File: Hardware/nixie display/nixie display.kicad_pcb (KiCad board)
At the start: 2 copper layers, 99.8 x 49.6 mm, 37 parts, among them J1 Conn_01x05_Male, J2 Conn_01x03_Male, J3 Conn_01x02_Male, J4 Conn_01x02_Male, J5 Conn_01x05_Male, J6 Conn_01x02_Male, Q1 MJE13003, Q2 Q_NMOS_GSD, U1 K155ID1, U10 TLP627, U7 TLP627, U8 TLP627, U9 TLP627

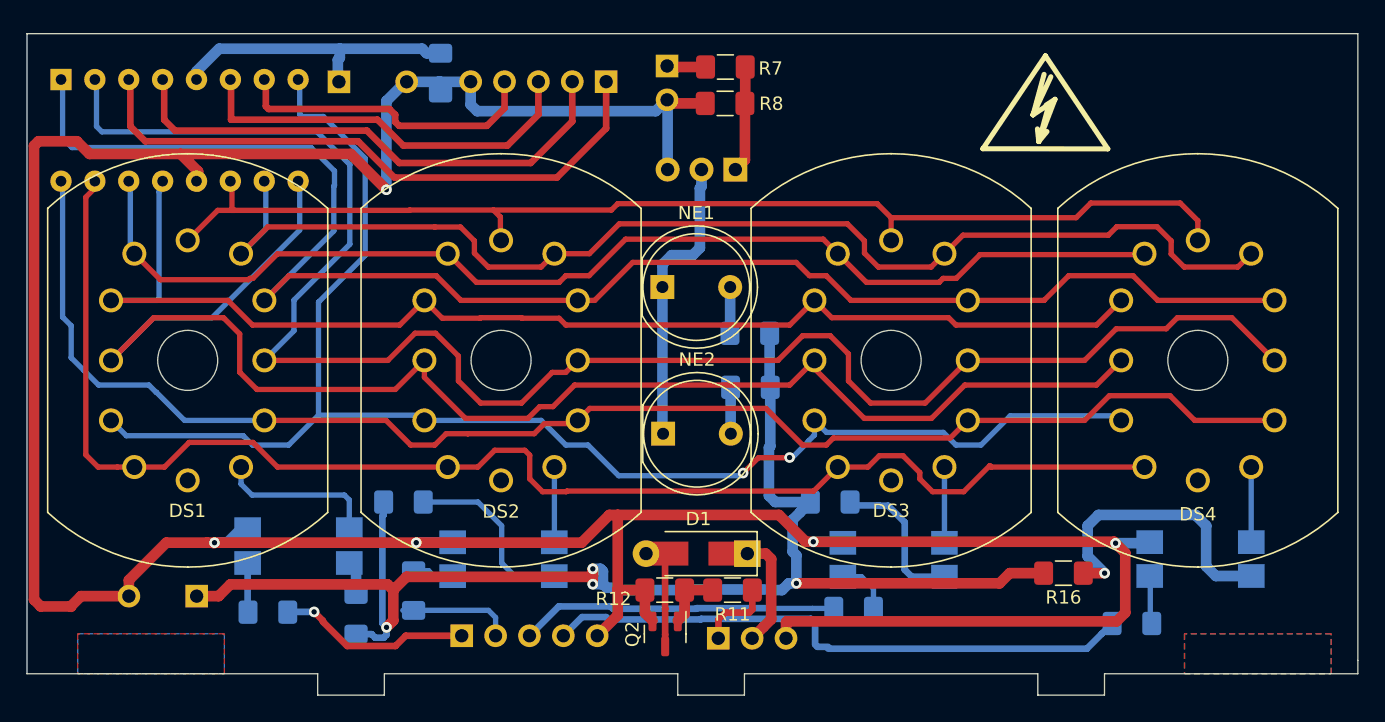
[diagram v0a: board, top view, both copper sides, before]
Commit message: Major HW and FW improvements
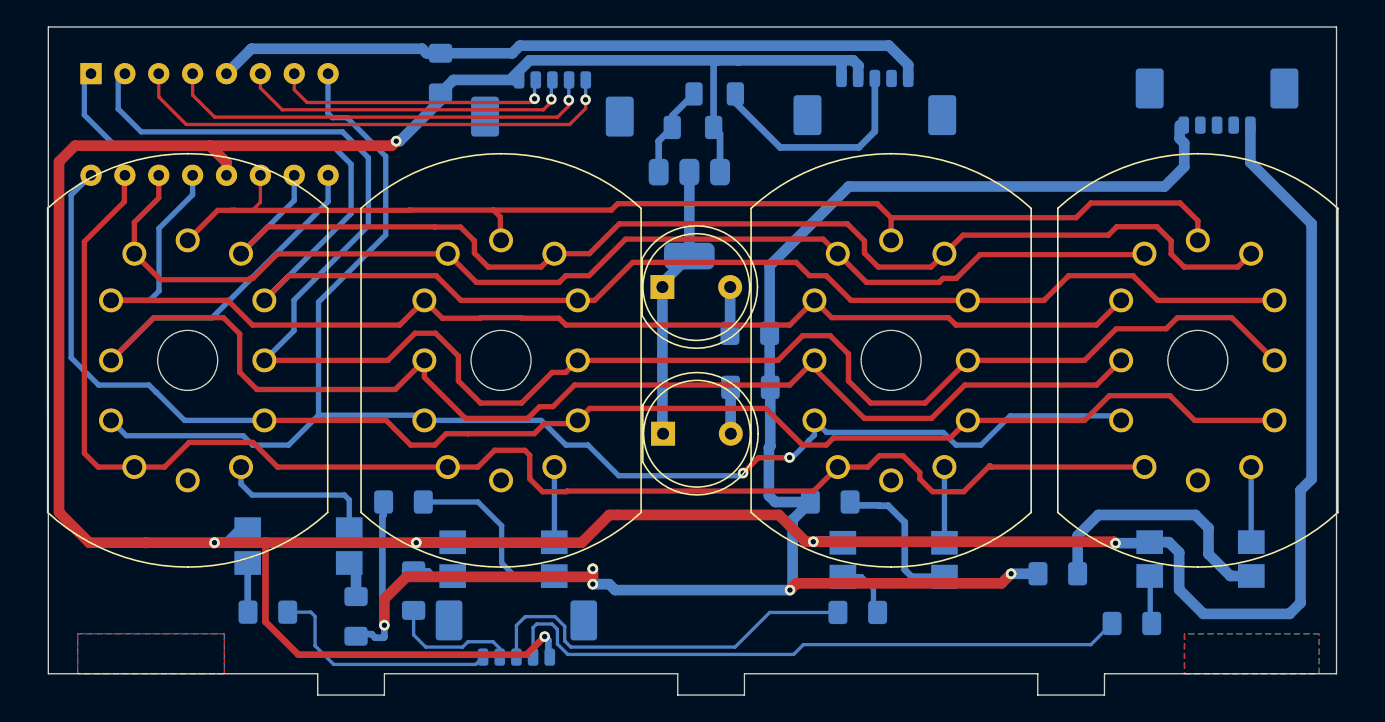
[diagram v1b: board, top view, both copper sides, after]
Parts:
- removed BZ1: Buzzer, Buzzer_Beeper:Buzzer_12x9.5RM7.6
- removed D1: SS14, Diode_SMD:D_SMA_Handsoldering
- removed J4, J6: Conn_01x02_Male, nixie clock:PinHeader_1x02_P5.08mm_Vertical
- removed Q2: Q_NMOS_GSD, Package_TO_SOT_SMD:SOT-23
- removed R11, R7: 100, Resistor_SMD:R_1206_3216Metric_Pad1.42x1.75mm_HandSolder
- removed R12, R8: 10k, Resistor_SMD:R_1206_3216Metric_Pad1.42x1.75mm_HandSolder
- removed REF**: HighVoltage, custom:HighVoltage
- added R1: 47k, Resistor_SMD:R_1206_3216Metric_Pad1.30x1.75mm_HandSolder, B.Cu at (160.1, 59.0)
- added R2: 100, Resistor_SMD:R_1206_3216Metric_Pad1.30x1.75mm_HandSolder, B.Cu at (161.8, 56.5)
- added SYM1: SYM_Flash_Large, custom:HighVoltage, B.Cu at (186.3, 64.1)
- J1, J5: value Conn_01x05_Male -> HCZZ0015-5; footprint Connector_PinHeader_2.54mm:PinHeader_1x05_P2.54mm_Vertical -> Connector_Molex:Molex_PicoBlade_53398-0571_1x05-1MP_P1.25mm_Vertical
- J2: value Conn_01x03_Male -> HCZZ0015-5; footprint Connector_PinHeader_2.54mm:PinHeader_1x03_P2.54mm_Vertical -> Connector_Molex:Molex_PicoBlade_53398-0571_1x05-1MP_P1.25mm_Vertical
- J3: value Conn_01x02_Male -> HCZZ0015-5; footprint Connector_PinHeader_2.54mm:PinHeader_1x02_P2.54mm_Vertical -> Connector_Molex:Molex_PicoBlade_53398-0571_1x05-1MP_P1.25mm_Vertical
- Q1: value MJE13003 -> FJT44; footprint Package_TO_SOT_THT:TO-126-3_Vertical -> Package_TO_SOT_SMD:SOT-223-3_TabPin2
- R10, R9: value 100k -> 47k
- R16: moved to B.Cu
- U1: value K155ID1 -> DS1009-16AT1NX-0A2
- moved J5 45.9 mm to (199.4, 57.6), turned to 0 degrees
- moved J2 42.5 mm to (149.6, 56.7), turned to 180 degrees
- moved J3 15.7 mm to (173.8, 56.6)
- moved Q1 4.80 mm to (159.9, 65.5), turned to -90 degrees
- moved J1 4.11 mm to (146.9, 97.5), turned to 0 degrees
- moved U1 2.29 mm to (115.0, 55.0)
- moved R19 0.43 mm to (172.5, 95.4)
- moved R16 0.43 mm to (187.5, 92.5)
- moved R13 0.16 mm to (134.9, 95.7)
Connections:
- J2 pad 1: Net-(J2-Pad1) -> /D0
- J2 pad 2: /V_Buzzer -> /D3
- J2 pad 3: GND -> /D1
- J3 pad 1: Net-(J3-Pad1) -> +5V
- J3 pad 2: GND -> unconnected-(J3-Pin_2-Pad2)
- J5 pad 1: /D0 -> VCC
- J5 pad 2: /D3 -> unconnected-(J5-Pin_2-Pad2)
- J5 pad 3: /D1 -> unconnected-(J5-Pin_3-Pad3)
- J5 pad 4: /D2 -> unconnected-(J5-Pin_4-Pad4)
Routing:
- net GND: track 247.6 -> 280.3 mm, vias 5 -> 6
- net +5V: track 22.3 -> 53.9 mm
- net VCC: track 108.8 -> 133.0 mm, vias 4 -> 5
- net Net-(J3-Pin_3): track 0.00 -> 17.0 mm
- net /V_Buzzer: track 9.66 -> 0.00 mm
- net /D0: track 45.4 -> 37.3 mm, vias 0 -> 1
- net Net-(BZ1-Pad2): track 7.02 -> 0.00 mm
- net /D3: track 38.8 -> 32.8 mm, vias 0 -> 1
- net Net-(J2-Pad1): track 5.66 -> 0.00 mm
- net /A3: track 23.8 -> 29.4 mm
- net Net-(Q2-Pad1): track 4.60 -> 0.00 mm
- net /D1: track 29.9 -> 25.5 mm, vias 0 -> 1
- net /A4: track 44.6 -> 48.3 mm
- net /A1: track 14.5 -> 17.8 mm, vias 1 -> 0
- net Net-(J3-Pad1): track 2.92 -> 0.00 mm
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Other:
- board size 99.8 x 49.6 mm -> 96.6 x 50.1 mm
- rule pad_to_mask_clearance: 0.051 -> 0
- board text added: "⎓250 V"
- board text removed: "+180V"
- board text removed: "+5V"
- board text removed: "A1"
- board text removed: "A2"
- board text removed: "A3"
- board text removed: "A4"
- board text removed: "D0"
- board text removed: "D1"
- board text removed: "D2"
- board text removed: "D3"
- board text removed: "GND"
- board text removed: "NE"
- board text removed: "S"
